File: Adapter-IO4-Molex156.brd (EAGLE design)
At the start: 30.9 x 31.9 mm, 3 parts

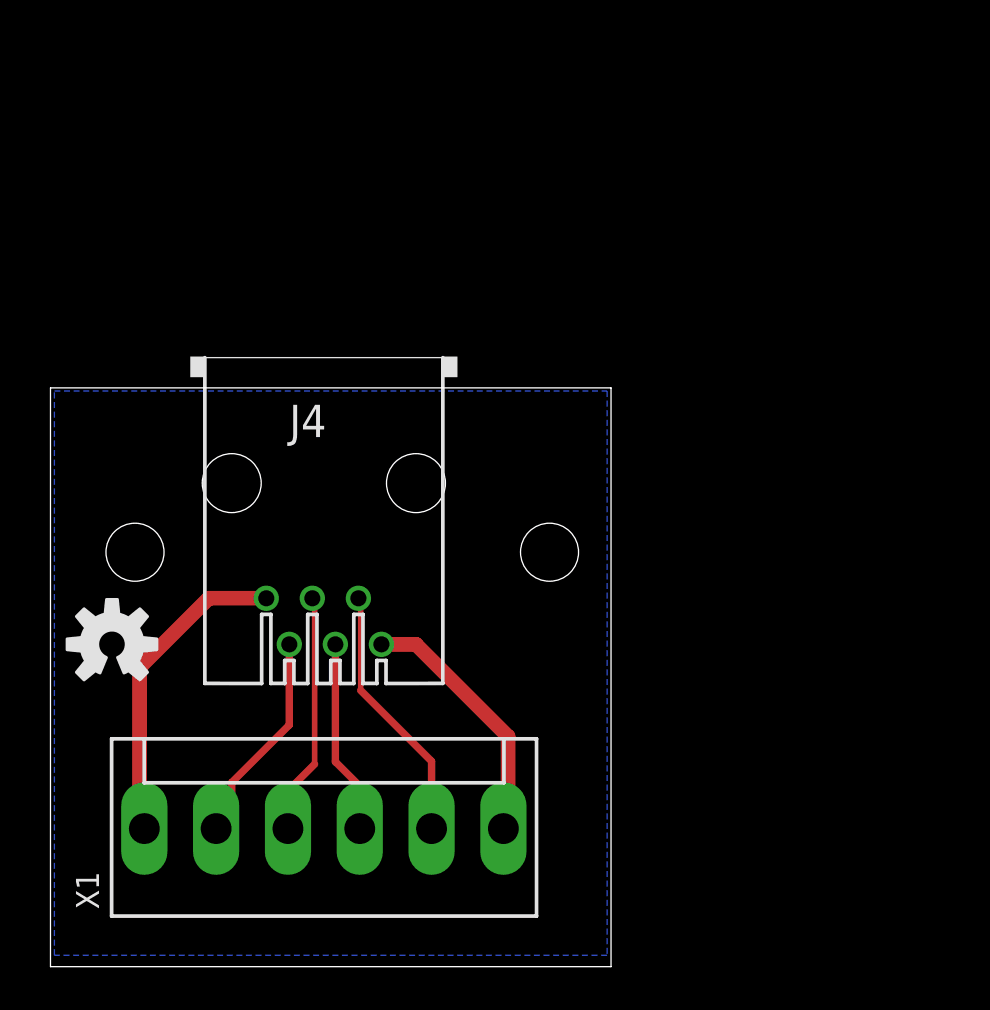
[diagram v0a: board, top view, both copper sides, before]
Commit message: 1.1
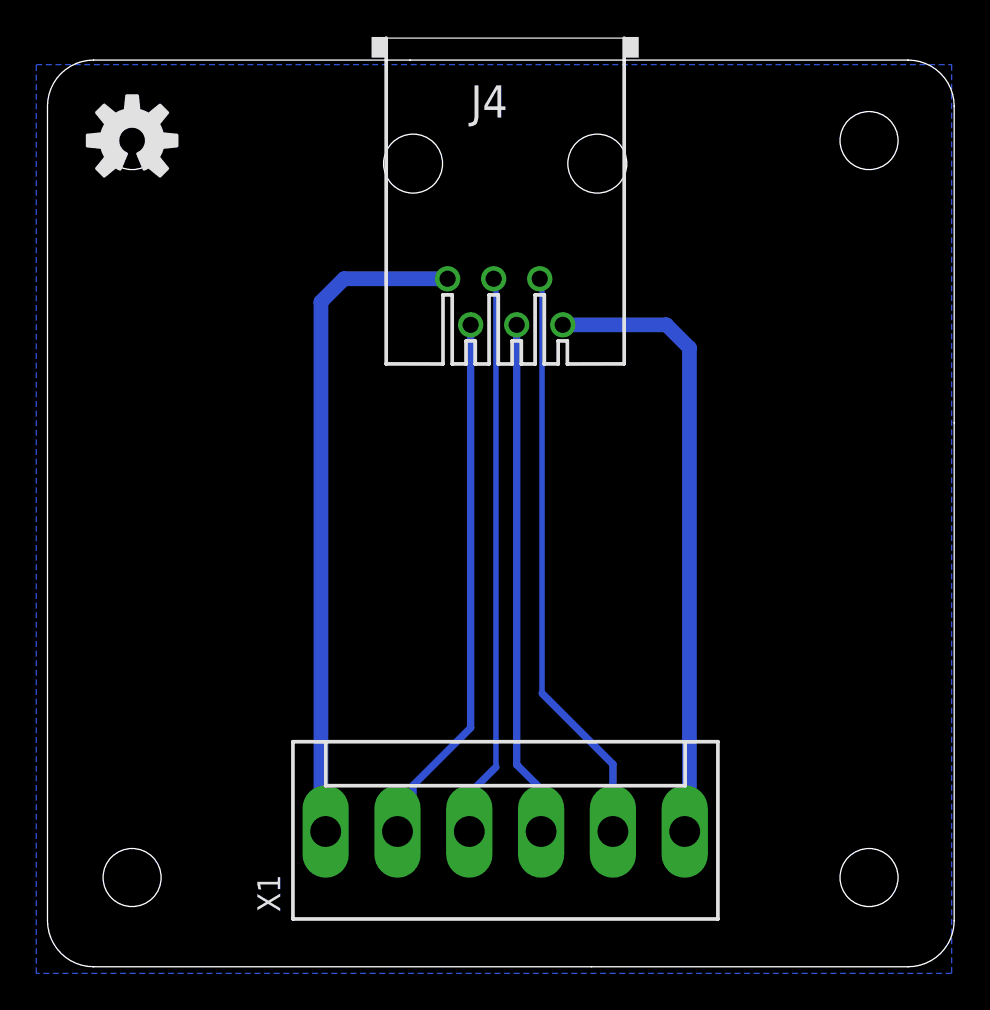
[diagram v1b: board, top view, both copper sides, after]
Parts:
- moved U$1 27.8 mm to (4.67, 45.6)
- moved J4 20.3 mm to (25.2, 44.3)
- moved X1 10.0 mm to (25.2, 7.46)
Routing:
- net VCC: track 14.3 -> 34.3 mm
- net GND: track 17.6 -> 36.8 mm
- net IO3: track 13.5 -> 31.2 mm, vias 0 -> 2
- net IO2: track 10.8 -> 28.5 mm
- net IO1: track 14.4 -> 32.2 mm
- net IO4: track 11.8 -> 29.6 mm
- added copper zone on layer 16, net GND
- removed copper zone on layer 16, net N$1
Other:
- board size 30.9 x 31.9 mm -> 50 x 50 mm
- board text added: "0.156 Pitch"
- board text added: "0.156 pitch"
- board text added: "2014.02"
- board text added: "IO4 Adapter"
- board text added: "IO4-Breakout"
- board text added: "v1.1"
- board text removed: "2012.08"
- board text removed: "Breakout"
- board text removed: "IOShield"
- board text removed: "IOShield Adapter"
- board text removed: "Lines"
- board text removed: "SPCoast"
- board text removed: "v1.0"
